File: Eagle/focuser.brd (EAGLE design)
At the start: 52 x 110.2 mm, 50 parts, among them IC1 78xx, J1 J5MM, J10 J5MM, J2 J7MM, J3 J7MM, J4 J5MM, J5 J7MM, J6 J12MM, J7 J7MM, J8 J7MM, J9 J5MM, U1 L298

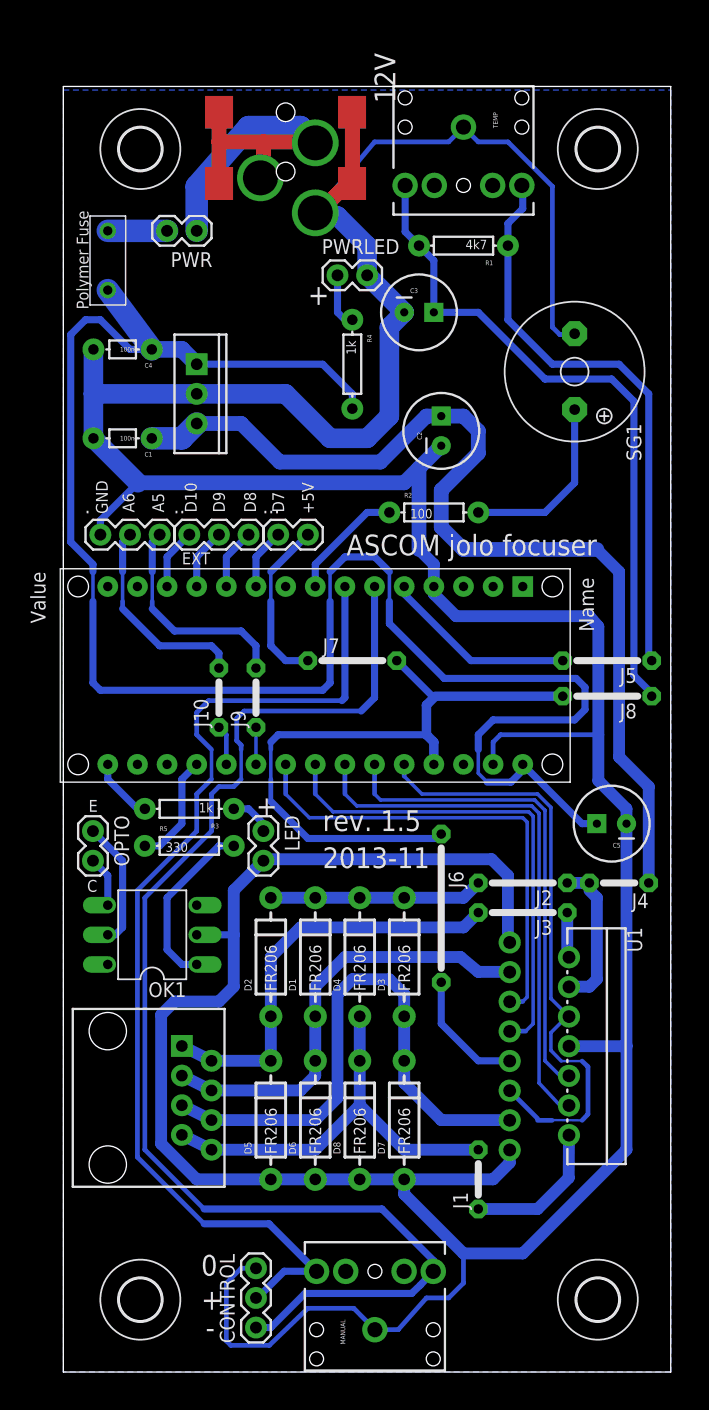
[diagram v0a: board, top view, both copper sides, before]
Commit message: Focuser 2.0
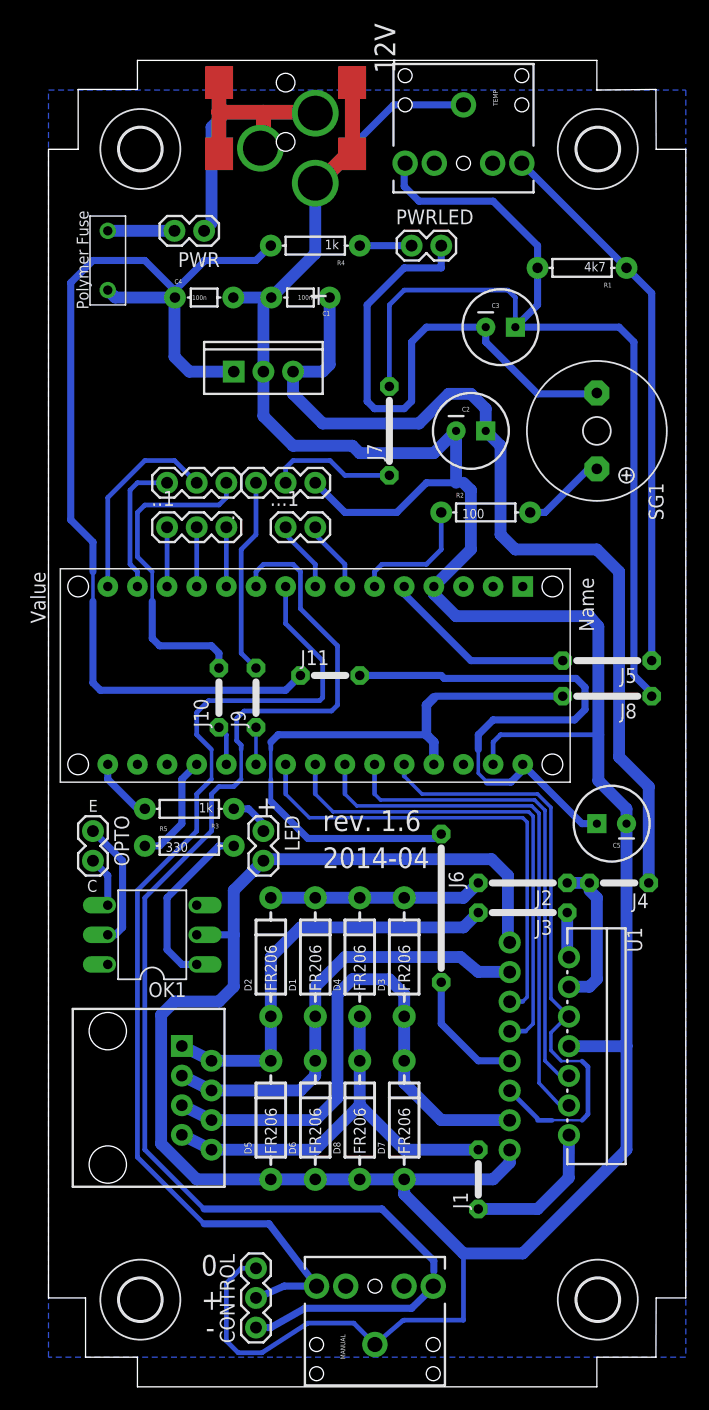
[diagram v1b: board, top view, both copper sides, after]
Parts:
- removed ...: (no value), SparkFun:1X02
- added ...1: (no value), SparkFun:1X02
- added ..1: (no value), SparkFun:1X03
- added J11: J5MM, jumper:05
- moved J7 19.9 mm to (27.9, 80.6), turned to 90 degrees
- moved C1 19.4 mm to (20.3, 92.1)
- moved . 18.9 mm to (21.6, 76.2), turned to 180 degrees
- moved R4 10.6 mm to (21.6, 96.5), turned to 180 degrees
- moved R1 10.3 mm to (44.5, 94.6)
- moved C4 8.28 mm to (12.1, 92.1), turned to 0 degrees
- moved C3 7.10 mm to (37.5, 89.5)
- moved PWRLED 6.84 mm to (29.8, 96.5)
- moved IC1 6.02 mm to (17.1, 85.7), turned to 0 degrees
- moved .. 5.46 mm to (14.0, 76.2), turned to 180 degrees
- moved SG1 5.43 mm to (45.7, 80.6)
- moved R2 4.45 mm to (36.2, 73.7)
- moved C2 2.54 mm to (34.9, 80.6), turned to 0 degrees
- moved 12V 2.54 mm to (19.1, 110.5)
- moved TEMP 1.90 mm to (34.3, 108.6)
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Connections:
- removed net N$30: C3.1, J8.1, R1.P$2, TEMP.5
- new net N$41: ..1.1, NANO.D10
- new net N$42: ...3, NANO.D11
- new net N$43: ...2, NANO.D12
- new net N$44: C5.1, J11.2, NANO.VIN
- new net N$45: J6.1, J8.2, NANO.+5V
- net +5: now also C3.1, J8.1, R1.P$2, TEMP.5; no longer J6.1, J8.2, NANO.+5V
- net N$18: now also NANO.D6; no longer NANO.D4
- net N$24: now also NANO.D7; no longer NANO.D3
- net N$31: now also ...1; no longer ..2
- net N$32: now also ...1.2, NANO.D4; no longer ...3, NANO.D8
- net N$33: now also ...1.1, NANO.D5; no longer ...2, NANO.D9
- net N$34: now also ..1.3, NANO.D8; no longer ...1, NANO.D10
- net N$35: now also ..1.2, NANO.D9; no longer NANO.D5, R2.P$1
- net N$6: now also ..2; no longer ....2
- net N$8: now also NANO.D3, R2.P$1; no longer ....1, NANO.D7
- net N$9: now also J11.1; no longer C5.1, NANO.VIN
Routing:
- net N$9: track 154.2 -> 91.6 mm
- net N$30: track 58.1 -> 0.00 mm
- net N$45: track 0.00 -> 52.2 mm
- net N$44: track 0.00 -> 48.5 mm
- net +5: track 56.7 -> 85.9 mm
- net N$43: track 0.00 -> 17.3 mm
- net N$42: track 0.00 -> 12.0 mm
- net N$31: track 17.7 -> 28.2 mm
- net GND: track 378.9 -> 369.9 mm
- net N$1: track 15.6 -> 7.26 mm
- net N$24: track 110.2 -> 116.0 mm
- net N$8: track 5.23 -> 10.9 mm
- net VCC2: track 86.1 -> 80.7 mm
- net N$41: track 0.00 -> 5.08 mm
- net N$35: track 10.1 -> 5.08 mm
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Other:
- board size 52 x 110.2 mm -> 54.6 x 113.7 mm
- board text added: "2014-04"
- board text added: "rev. 1.6"
- board text removed: "+5V"
- board text removed: "2013-11"
- board text removed: "A5"
- board text removed: "A6"
- board text removed: "ASCOM jolo focuser"
- board text removed: "D10"
- board text removed: "D7"
- board text removed: "D8"
- board text removed: "D9"
- board text removed: "EXT"
- board text removed: "GND"
- board text removed: "rev. 1.5"
